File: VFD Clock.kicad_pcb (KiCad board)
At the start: 2 copper layers, 224 x 78 mm, 41 parts, among them J2 Mode Button, J3 Up Button, J4 Down Button, J5 Select Button, U1 74HC595, U10 74HC595, U11 UDN2981A, U12 Minute Right, U13 74HC595, U14 UDN2981A, U15 Second Left, U16 74HC595, U17 UDN2981A, U18 Second Right, U19 XL6009 Module, U2 UDN2981A, U20 LM2596 Module, U21 DS3231 Module, U3 Hour Left, U4 74HC595, U5 UDN2981A, U6 Hour Right, U7 74HC595, U8 UDN2981A, U9 Minute Left

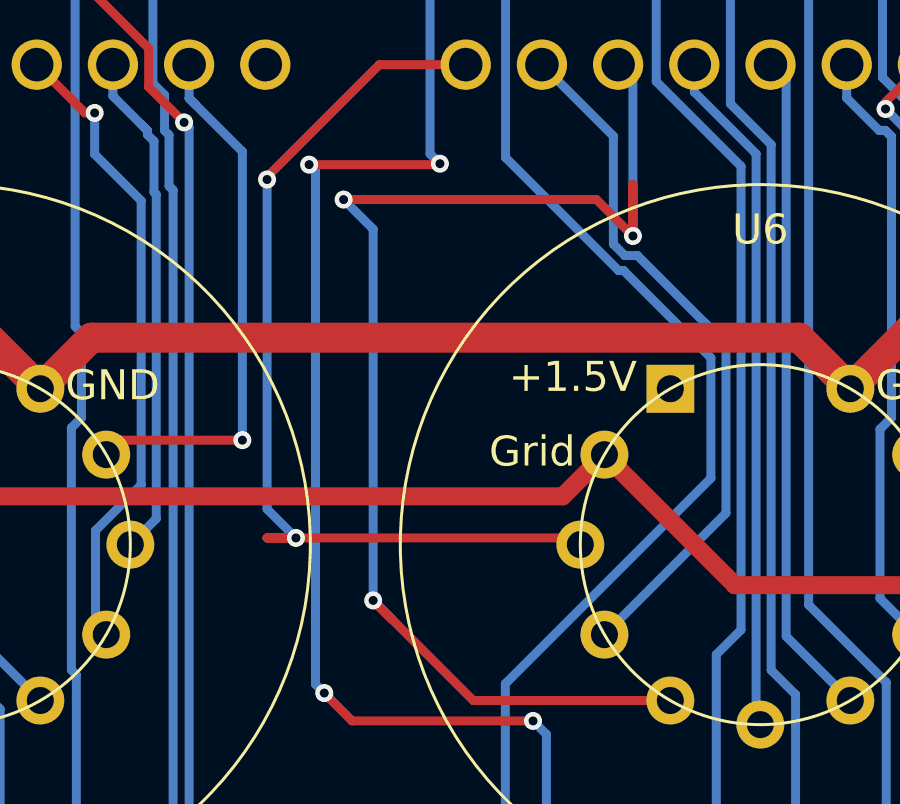
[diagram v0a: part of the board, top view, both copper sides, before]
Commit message: save
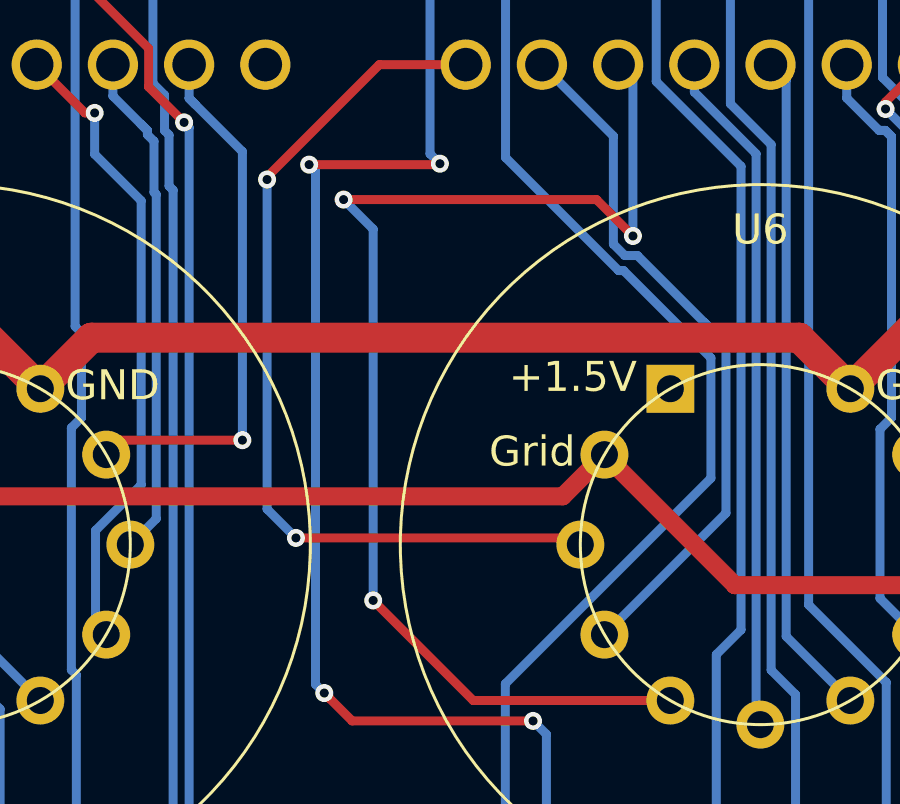
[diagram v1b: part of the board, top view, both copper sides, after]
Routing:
- net Net-(U5-OUT3): track 51.8 -> 41.4 mm
- net Net-(U5-OUT1): track 34.0 -> 30.2 mm
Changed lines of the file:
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@@
 		)
 		(property "Value" "74HC595"
-			(at 9.807294 -16 0)
+			(at 9.59 -15.93 0)
 			(layer "B.SilkS")
 			(effects
@@
 		)
 		(property "Value" "74HC595"
-			(at 10 -16 0)
+			(at 9.64 -15.89 0)
 			(layer "B.SilkS")
 			(effects
@@
 			(at 1.25 2.05 0)
 			(layer "B.SilkS")
+			(hide yes)
 			(effects
 				(font
@@
 			(at 1.25 2.05 0)
 			(layer "B.SilkS")
+			(hide yes)
 			(effects
 				(font
@@
 			(at 1.25 2.05 0)
 			(layer "B.SilkS")
+			(hide yes)
 			(effects
 				(font
@@
 		(tags "C Disc series Radial pin pitch 2.50mm diameter 3.0mm width 1.6mm Capacitor")
 		(property "Reference" "C16"
-			(at 1.25 2.05 0)
+			(at -2.5 -0.5 0)
 			(layer "B.SilkS")
+			(hide yes)
 			(effects
 				(font
@@
 	)
 	(segment
-		(start 110.5581 99.7768)
-		(end 111.5203 99.7768)
-		(width 0.3)
-		(layer "F.Cu")
-		(net "Net-(U5-OUT1)")
-	)
-	(segment
 		(start 111.5203 99.7768)
 		(end 120.7768 99.7768)
@@
 	)
 	(segment
-		(start 111.5203 99.7768)
-		(end 110.5581 99.7768)
-		(width 0.3)
-		(layer "F.Cu")
-		(net "Net-(U5-OUT1)")
-	)
-	(segment
 		(start 120.7768 99.7768)
 		(end 121 100)
@@
 	)
 	(segment
-		(start 111.5203 99.7768)
-		(end 110.5581 99.7768)
-		(width 0.3)
-		(layer "B.Cu")
-		(net "Net-(U5-OUT1)")
-	)
-	(segment
-		(start 110.5581 99.7768)
-		(end 111.5203 99.7768)
-		(width 0.3)
-		(layer "B.Cu")
-		(net "Net-(U5-OUT1)")
-	)
-	(segment
 		(start 110.5581 98.8146)
 		(end 110.5581 87.8295)
@@
 	)
 	(segment
-		(start 114.0948 101.8602)
-		(end 114.7199 102.4853)
-		(width 0.3)
-		(layer "F.Cu")
-		(net "Net-(U5-OUT3)")
-	)
-	(segment
-		(start 114.7199 102.4853)
-		(end 114.0948 101.8602)
-		(width 0.3)
-		(layer "F.Cu")
-		(net "Net-(U5-OUT3)")
-	)
-	(segment
 		(start 121.5401 88.4984)
 		(end 122.7537 89.712)
@@
 	)
 	(segment
-		(start 122.7537 87.9957)
-		(end 122.7537 89.712)
-		(width 0.3)
-		(layer "F.Cu")
-		(net "Net-(U5-OUT3)")
-	)
-	(segment
-		(start 122.7537 89.712)
-		(end 122.7537 87.9957)
-		(width 0.3)
-		(layer "F.Cu")
-		(net "Net-(U5-OUT3)")
-	)
-	(segment
 		(start 117.4307 105.1961)
 		(end 114.0948 101.8602)
@@
 	)
 	(segment
-		(start 114.0948 101.8602)
-		(end 114.7199 102.4853)
-		(width 0.3)
-		(layer "B.Cu")
-		(net "Net-(U5-OUT3)")
-	)
-	(segment
 		(start 113.1092 88.4984)
 		(end 113.188 88.4984)
@@
 	)
 	(segment
-		(start 122.7537 87.9957)
-		(end 122.7537 89.712)
-		(width 0.3)
-		(layer "B.Cu")
-		(net "Net-(U5-OUT3)")
-	)
-	(segment
 		(start 122.7537 89.712)
 		(end 122.7537 84.4937)
@@
 	)
 	(segment
-		(start 122.7537 89.712)
-		(end 122.7537 87.9957)
-		(width 0.3)
-		(layer "B.Cu")
-		(net "Net-(U5-OUT3)")
-	)
-	(segment
-		(start 114.7199 102.4853)
-		(end 114.0948 101.8602)
-		(width 0.3)
-		(layer "B.Cu")
-		(net "Net-(U5-OUT3)")
-	)
-	(segment
 		(start 122.7537 84.4937)
 		(end 122.26 84)
@@
 		(name "Ground Pour")
 		(hatch none 0.5)
-		(connect_pads
+		(connect_pads yes
 			(clearance 0.25)
 		)
 		(min_thickness 0.25)
 		(fill yes
-			(thermal_gap 0.4)
+			(thermal_gap 0.25)
 			(thermal_bridge_width 0.25)
-			(smoothing chamfer)
+			(smoothing fillet)
 			(radius 0.5)
 			(island_removal_mode 0)
